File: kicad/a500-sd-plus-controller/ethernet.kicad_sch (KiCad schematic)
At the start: 24 parts, among them J5 RJ45, U10 ENC28J60x-SS, Y2 25.0MHz

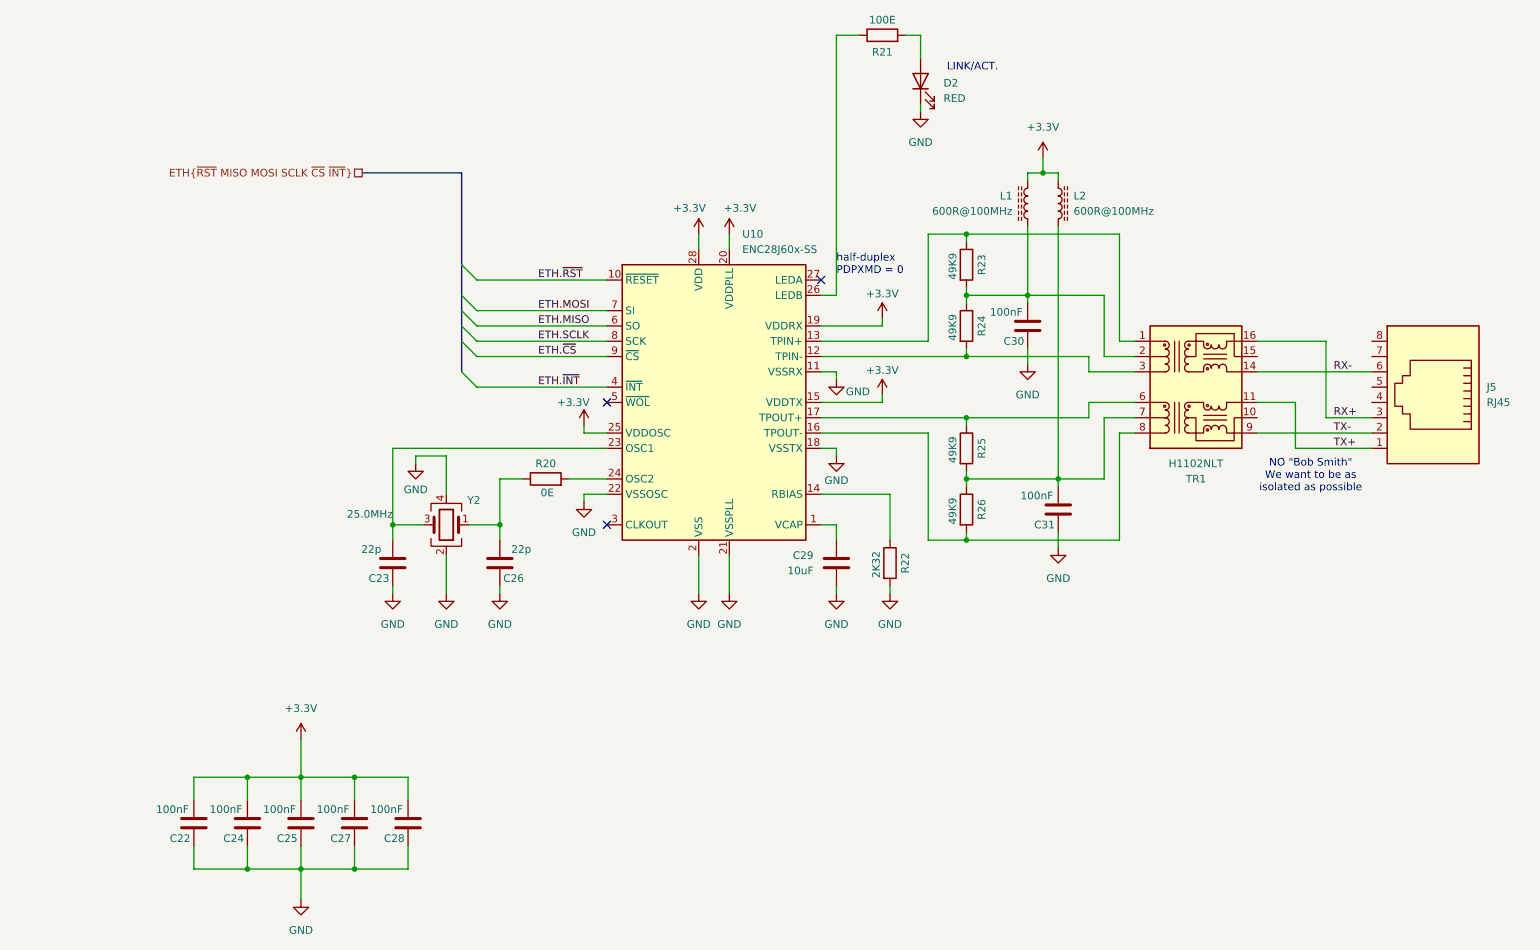
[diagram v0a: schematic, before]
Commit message: PCB done, this version has been sent to fabrication
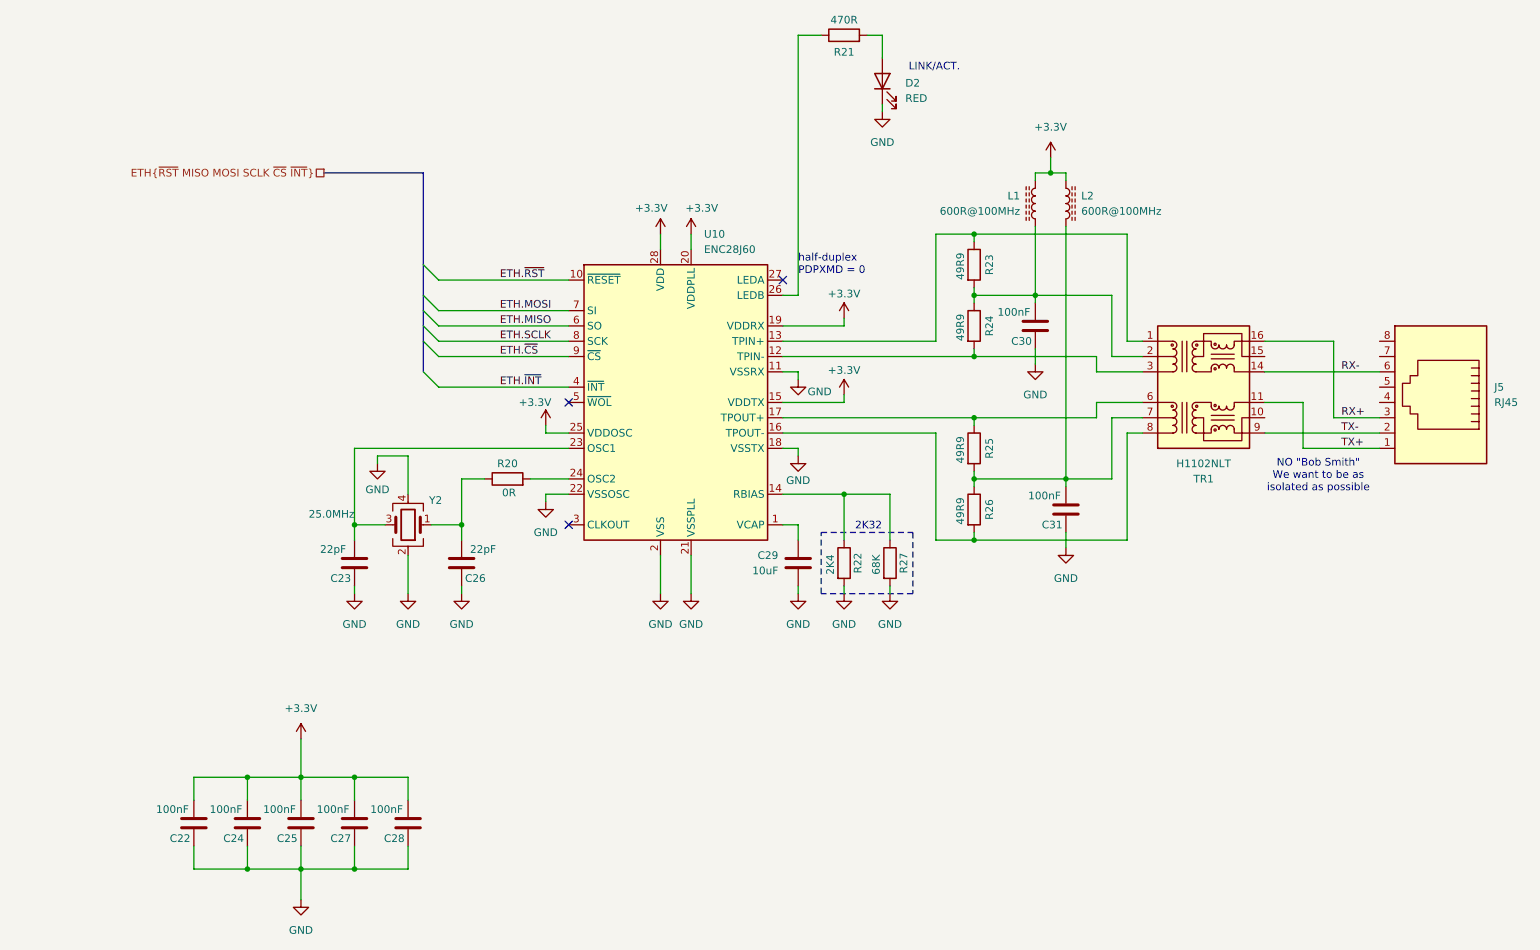
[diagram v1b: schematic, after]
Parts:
- added R27: 68K, Resistor_SMD:R_0603_1608Metric, symbol Device:R
- C22, C24, C25, C27, C28, C30, C31: LCSC Part # (none) -> C14663; Quantity (none) -> ${QUANTITY}
- C23, C26: value 22p -> 22pF; LCSC Part # (none) -> C1653; Quantity (none) -> ${QUANTITY}
- C29: LCSC Part # (none) -> C15850; Quantity (none) -> ${QUANTITY}
- D2: LCSC Part # (none) -> C84256; Quantity (none) -> ${QUANTITY}
- J5: LCSC Part # (none) -> C385834; Quantity (none) -> ${QUANTITY}
- L1, L2: LCSC Part # (none) -> C1017; Quantity (none) -> ${QUANTITY}
- R20: value 0E -> 0R; LCSC Part # (none) -> C21189; Quantity (none) -> ${QUANTITY}
- R21: value 100E -> 470R; LCSC Part # (none) -> C23179; Quantity (none) -> ${QUANTITY}
- R22: value 2K32 -> 2K4; LCSC Part # (none) -> C22940; Quantity (none) -> ${QUANTITY}
- R23, R24, R25, R26: value 49K9 -> 49R9; LCSC Part # (none) -> C23185; Quantity (none) -> ${QUANTITY}
- TR1: LCSC Part # (none) -> C18584; MPN (none) -> H1102NLT; Quantity (none) -> ${QUANTITY}
- U10: value ENC28J60x-SS -> ENC28J60; LCSC Part # (none) -> C411626; MPN (none) -> ENC28J60-I/SS; Quantity (none) -> ${QUANTITY}
- Y2: LCSC Part # (none) -> C9006; Quantity (none) -> ${QUANTITY}
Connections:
- net GND: now also R27.2
- net at R22.1, U10.14 (RBIAS): now also R27.1
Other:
- note added: "2K32"
- moved on the sheet: C23, C26, C29, C30, C31, D2, J5, L1, L2, R20, R21, R22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
